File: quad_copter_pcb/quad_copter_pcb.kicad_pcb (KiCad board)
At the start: 2 copper layers, 111.8 x 108.1 mm, 68 parts, among them J1 Conn_01x03_Male, J10 Conn_02x03_Odd_Even, J11 Conn_01x05, J12 USB_B_Micro, J2 Conn_01x03_Male, J3 Conn_01x03_Male, J4 Conn_01x03_Male, J5 Conn_02x05_Odd_Even, J6 Conn_02x02_Odd_Even, J7 Conn_01x05, J8 Conn_02x04_Odd_Even, J9 Conn_02x02_Odd_Even, U1 LT1085-3.3, U3 accel_gyro_conn, U4 PIC32MX795F512L-X_PT, Y1 Crystal_8MHz, Y2 Crystal_GND23

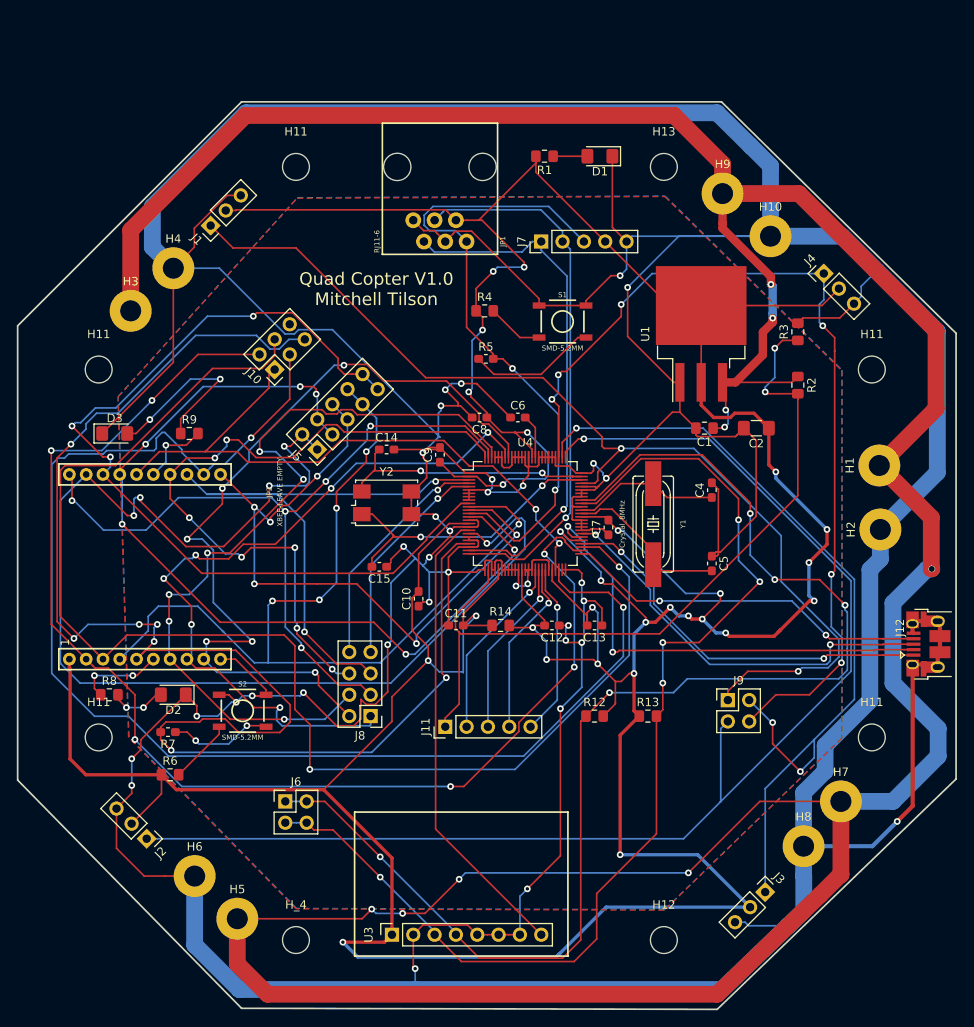
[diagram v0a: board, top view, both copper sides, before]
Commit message: PCB updates
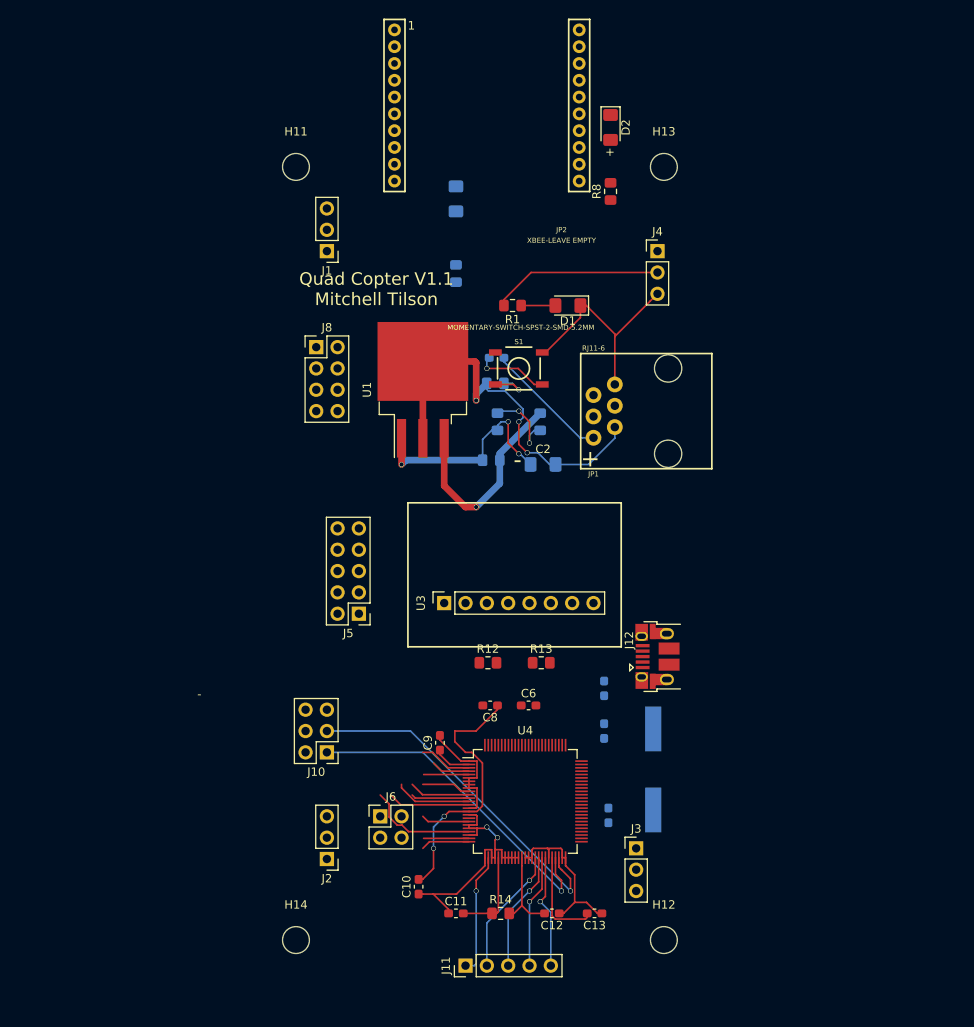
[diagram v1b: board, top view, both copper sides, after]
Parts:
- removed C14, C15: C15pF, Capacitor_SMD:C_0603_1608Metric_Pad1.05x0.95mm_HandSolder
- removed H1, H10, H2, H3, H4, H5, H6, H7, H8, H9: MountingHole_Pad, MountingHole:MountingHole_2.5mm_Pad
- removed the H11 at (191.9, 71.2)
- removed the H11 at (191.9, 115.1)
- removed the H11 at (99.8, 115.1)
- removed the H11 at (99.8, 71.2)
- removed J7: Conn_01x05, Connector_PinHeader_2.54mm:PinHeader_1x05_P2.54mm_Vertical
- removed J9: Conn_02x02_Odd_Even, Connector_PinHeader_2.54mm:PinHeader_2x02_P2.54mm_Vertical
- removed R6: R10k, Resistor_SMD:R_0805_2012Metric_Pad1.15x1.40mm_HandSolder
- removed R7: R470, Resistor_SMD:R_0603_1608Metric_Pad1.05x0.95mm_HandSolder
- removed S2: SMD-5.2MM, Switches:TACTILE_SWITCH_SMD_5.2MM
- removed Y2: Crystal_GND23, Crystal:Crystal_SMD_7050-4Pin_7.0x5.0mm
- C1, C2, C4, C5, C7, D3, R2, R3, R4, R5, R9, Y1: moved to B.Cu
- S1: value SMD-5.2MM -> MOMENTARY-SWITCH-SPST-2-SMD-5.2MM
- moved D2 85.3 mm to (160.8, 42.4), turned to 270 degrees
- moved R8 84.6 mm to (160.8, 50.0), turned to 90 degrees
- moved JP2 53.0 mm to (146.1, 50.8), turned to 0 degrees
- moved D3 49.3 mm to (142.4, 50.9), turned to 270 degrees
- moved J10 46.0 mm to (127.0, 116.8), turned to 180 degrees
- moved J8 44.4 mm to (125.7, 68.6), turned to 0 degrees
- moved U3 40.0 mm to (141.0, 99.1)
- moved JP1 39.8 mm to (167.6, 76.2), turned to 90 degrees
- moved R3 37.3 mm to (147.3, 77.5), turned to 270 degrees
- moved R9 37.0 mm to (142.4, 59.8), turned to 270 degrees
- moved C6 34.3 mm to (151.0, 111.3)
- moved C8 34.3 mm to (146.4, 111.3)
- moved C10 34.3 mm to (137.9, 132.8)
- moved C9 34.3 mm to (140.5, 115.7)
- moved U4 34.3 mm to (150.6, 122.7)
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- renumbered H_4 to H14
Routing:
- net GND: track 916.7 -> 119.4 mm, vias 35 -> 5
- net VDD3.3: track 560.4 -> 137.5 mm, vias 28 -> 5
- net VBATT: track 418.1 -> 24.9 mm, vias 9 -> 1
- net XBEE_RESET: track 173.9 -> 13.3 mm, vias 7 -> 0
- net U1TX: track 157.9 -> 0.00 mm, vias 2 -> 0
- net I2C1_SDA1: track 156.8 -> 0.00 mm, vias 5 -> 0
- net MOTOR2_PWM: track 155.2 -> 0.00 mm, vias 1 -> 0
- net U1RX: track 151.4 -> 0.00 mm, vias 6 -> 0
- net SPI_ATTN_INT_L: track 146.8 -> 5.75 mm, vias 5 -> 0
- net I2C1_SCL1: track 132.2 -> 0.00 mm, vias 5 -> 0
- net MOTOR1_PWM: track 124.2 -> 0.00 mm, vias 2 -> 0
- net U1RTS: track 160.1 -> 41.4 mm, vias 2 -> 1
- net MOTOR4_PWM: track 110.0 -> 0.00 mm, vias 6 -> 0
- net SDI2_MISO_2: track 110.6 -> 7.27 mm, vias 5 -> 0
- net MOTOR3_PWM: track 102.0 -> 0.00 mm, vias 3 -> 0
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- removed copper zone on B.Cu, net GND
- removed copper zone on F.Cu, net VDD3.3
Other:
- board outline removed
- net class Default: clearance 0.2 -> 0.1
- rule trace_clearance: 0.2 -> 0.1
- board text added: "+"
- board text added: "-"
- board text added: "Quad Copter V1.1 Mitchell Tilson"
- board text removed: "Quad Copter V1.0 Mitchell Tilson"
